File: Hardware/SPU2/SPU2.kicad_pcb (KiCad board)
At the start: 2 copper layers, 736 parts, among them J1 Conn_Coaxial, J2 Conn_02x13_Counter_Clockwise, J3 Conn_01x02, J4 Conn_01x04_Male, Q2 BC547, Q3 BC547, Q4 BC547, SW1 SW_Push, SW2 SW_SPDT, SW3 SW_DIP_x02, U1 74LS86, U10 74LS08, U11 74LS173, U12 74LS173, U13 74LS161, U14 74LS161, U15 74LS161, U16 74LS173, U17 74LS173, U18 NE555, U19 74LS173, U2 74LS86, U20 74LS173, U21 74LS173, U22 74LS173, U23 74LS173, U24 74LS173, U25 74LS245, U26 M84Z02, U27 M84Z02, U28 74LS245, U29 74LS00, U3 74LS245, U30 28c64, U31 28c64, U32 74LS245, U33 74LS245, U34 74LS245, U35 74LS245, U36 74LS245, U37 74LS08, U38 74HCT574, U39 74HCT574, U4 74LS283, U40 74LS161, U41 74LS04, U42 74LS08, U43 NE555, U44 NE555, U45 74HCT574, U46 74HCT574, U47 74HCT574, U48 74HCT574, U49 74HCT574, U5 74LS283, U50 74HCT574, U51 74HCT574, U52 74HCT574, U53 74HCT574, U54 74HCT574, U55 74HCT574, U56 74HCT574, U57 74HCT574, U58 74HCT574, U59 74HCT574, U6 4077, U60 74HCT574, U61 INTEL2716, U62 74LS08, U63 INTEL2716, U64 74LS08, U65 74LS08, U66 74LS08, U67 74LS08, U68 INTEL2716, U69 CD4514B, U7 4077, U70 74LS157, U71 74LS245, U72 74LS245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

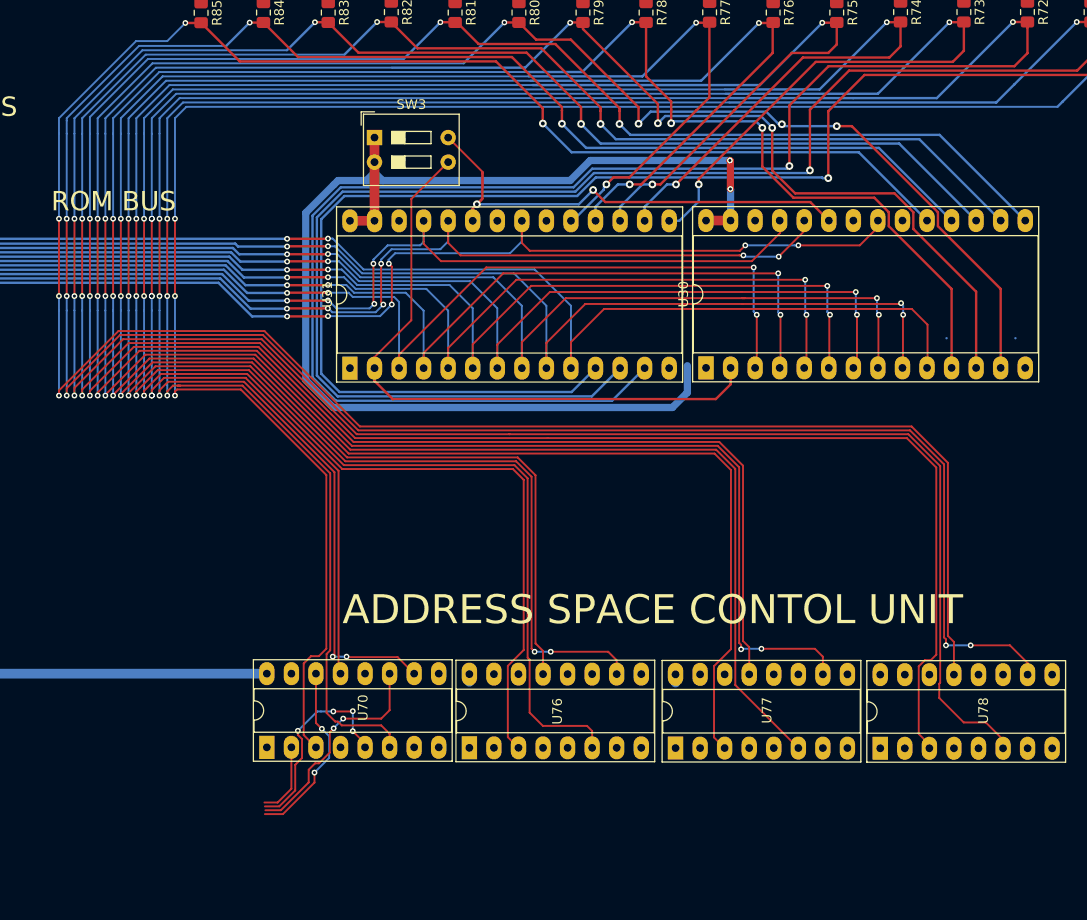
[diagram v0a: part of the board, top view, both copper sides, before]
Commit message: random push
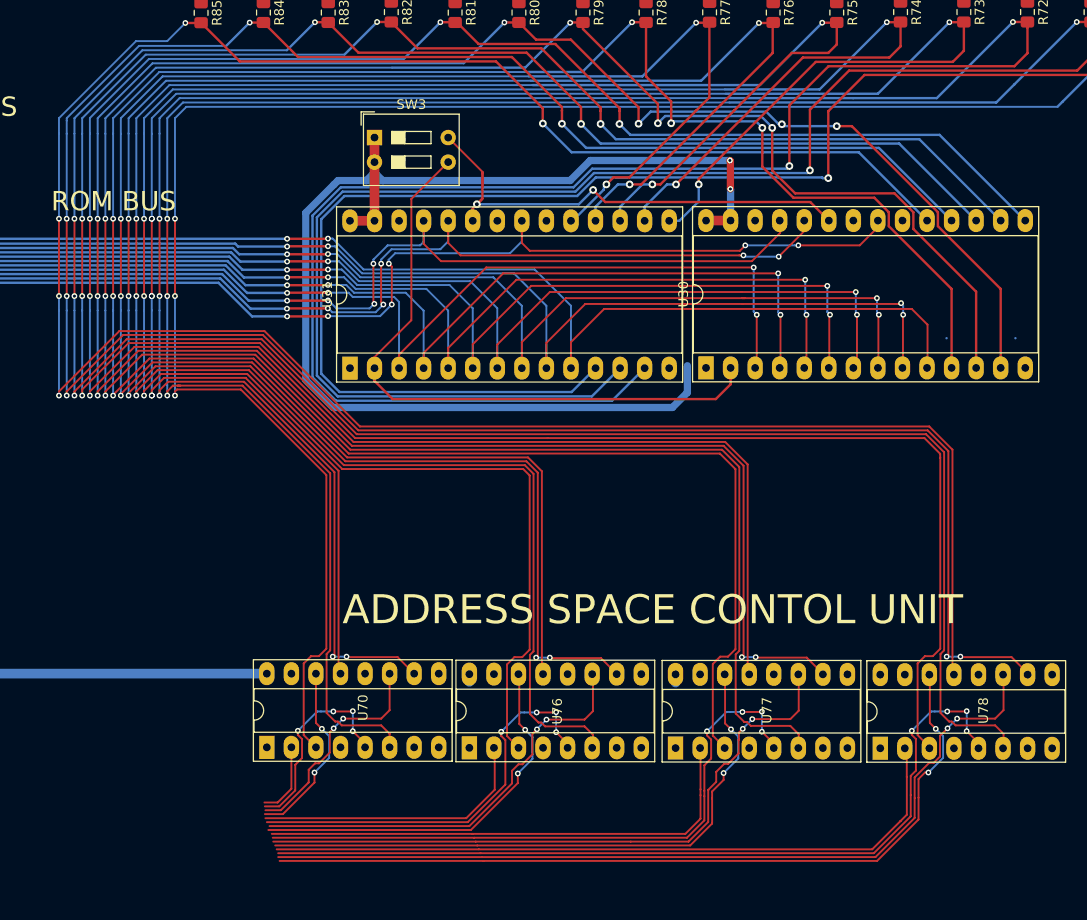
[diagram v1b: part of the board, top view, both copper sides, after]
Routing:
- net /RAMOBUS14: track 0.00 -> 88.8 mm, vias 0 -> 2
- net /RAMOBUS13: track 0.00 -> 87.0 mm, vias 0 -> 4
- net /RAMOBUS15: track 0.00 -> 84.8 mm, vias 0 -> 2
- net /RAMOBUS12: track 0.00 -> 73.7 mm
- net /RAMOBUS10: track 0.00 -> 67.5 mm, vias 0 -> 2
- net /RAMOBUS9: track 0.00 -> 65.9 mm, vias 0 -> 4
- net /RAMOBUS11: track 0.00 -> 63.3 mm, vias 0 -> 2
- net /RAMOBUS8: track 0.00 -> 52.3 mm
- net /RAMOBUS6: track 0.00 -> 44.2 mm, vias 0 -> 2
- net /RAMOBUS5: track 0.00 -> 42.7 mm, vias 0 -> 4
- net /RAMOBUS7: track 0.00 -> 40.2 mm, vias 0 -> 2
- net /RAMOBUS4: track 0.00 -> 29.2 mm
- net /ROM9: track 251.6 -> 255.0 mm
- net /ROM13: track 266.9 -> 270.0 mm
- net /ROM12: track 264.4 -> 266.3 mm
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
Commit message: done stuff
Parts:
- moved R62 423.1 mm to (327.1, 121.9), turned to 270 degrees
- moved D64 397.5 mm to (333.6, 115.5), turned to 270 degrees
- moved R264 387.8 mm to (359.8, 121.9), turned to 270 degrees
- moved D255 387.3 mm to (366.4, 115.5), turned to 270 degrees
- moved U33 371.7 mm to (509.4, 196.7)
- moved U32 370.5 mm to (499.1, 195.4)
- moved R63 366.1 mm to (386.1, 121.9), turned to 270 degrees
- moved R69 359.6 mm to (405.7, 121.9), turned to 270 degrees
- moved R66 349.9 mm to (340.2, 121.9), turned to 270 degrees
- moved D65 348.6 mm to (392.6, 115.5), turned to 270 degrees
- moved U27 347.9 mm to (396.4, 175.2), turned to 180 degrees
- moved U29 339.2 mm to (413.6, 168.2), turned to 180 degrees
- moved R268 319.7 mm to (372.9, 121.9), turned to 270 degrees
- moved R68 319.1 mm to (346.7, 121.9), turned to 270 degrees
- moved U26 316.2 mm to (369.9, 175.5), turned to 180 degrees
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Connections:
- D122 pad 1: Net-(D122-Pad1) -> GND
- D123 pad 1: Net-(D123-Pad1) -> GND
- D124 pad 1: Net-(D124-Pad1) -> GND
- D125 pad 1: Net-(D125-Pad1) -> GND
- D126 pad 1: Net-(D126-Pad1) -> GND
- D127 pad 1: Net-(D127-Pad1) -> GND
- D128 pad 1: Net-(D128-Pad1) -> GND
- D129 pad 1: Net-(D129-Pad1) -> GND
- D178 pad 1: Net-(D178-Pad1) -> GND
- D179 pad 1: Net-(D178-Pad1) -> GND
- D180 pad 1: Net-(D178-Pad1) -> GND
- D181 pad 1: Net-(D178-Pad1) -> GND
- D183 pad 1: Net-(D178-Pad1) -> GND
- D185 pad 1: Net-(D178-Pad1) -> GND
- D187 pad 1: Net-(D178-Pad1) -> GND
- D189 pad 1: Net-(D178-Pad1) -> GND
- U36 pad 6: /MEM12 -> GND
- U36 pad 7: /MEM13 -> GND
- U36 pad 8: /MEM14 -> GND
- U36 pad 9: /MEM15 -> GND
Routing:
- net +5V: track 753.1 -> 1590.7 mm, vias 11 -> 26
- net /RAMOBUS0: track 7.67 -> 231.8 mm, vias 0 -> 2
- net /MEMADDR0: track 355.0 -> 576.9 mm, vias 8 -> 12
- net CLK: track 193.1 -> 414.7 mm, vias 5 -> 8
- net /MEMADDR1: track 343.9 -> 557.7 mm, vias 12 -> 16
- net /RAMOBUS1: track 21.2 -> 233.4 mm, vias 4 -> 6
- net /MEMADDR2: track 330.0 -> 535.9 mm, vias 12 -> 16
- net /MEM11: track 0.00 -> 205.5 mm, vias 0 -> 2
- net /RAMOBUS2: track 22.9 -> 226.3 mm, vias 2 -> 4
- net /MEMADDR3: track 314.6 -> 512.0 mm, vias 12 -> 16
- net /MEM10: track 0.00 -> 197.2 mm
- net /RAMOBUS3: track 18.9 -> 212.1 mm, vias 2 -> 4
- net /RAMOBUS5: track 42.7 -> 235.4 mm, vias 4 -> 6
- net /MEMADDR4: track 275.5 -> 465.2 mm, vias 12 -> 16
- net /RAMOBUS4: track 29.2 -> 217.8 mm, vias 0 -> 2
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- added copper zone on B.Cu, net +5V
- added copper zone on B.Cu, net GND
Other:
- board outline added: 400 x 300 mm
- board text added: "RANDOM ACCESS MEMORY"
